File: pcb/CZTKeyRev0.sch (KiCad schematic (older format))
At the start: 268 parts, among them U1 proton_c

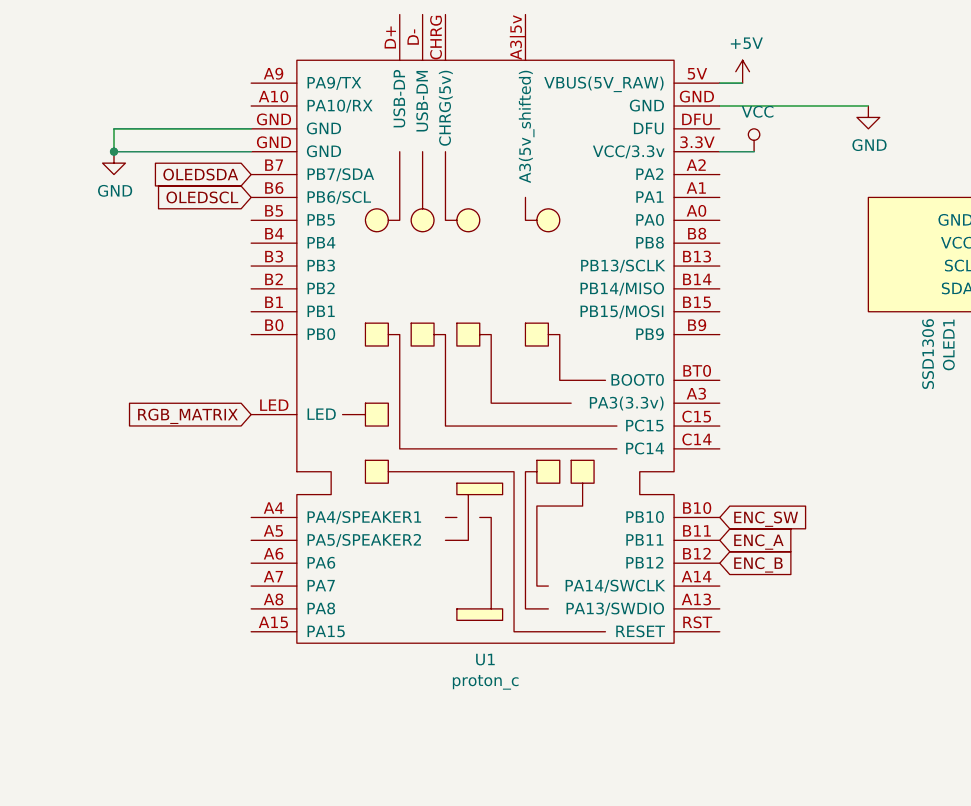
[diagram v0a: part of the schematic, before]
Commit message: Maybe final?
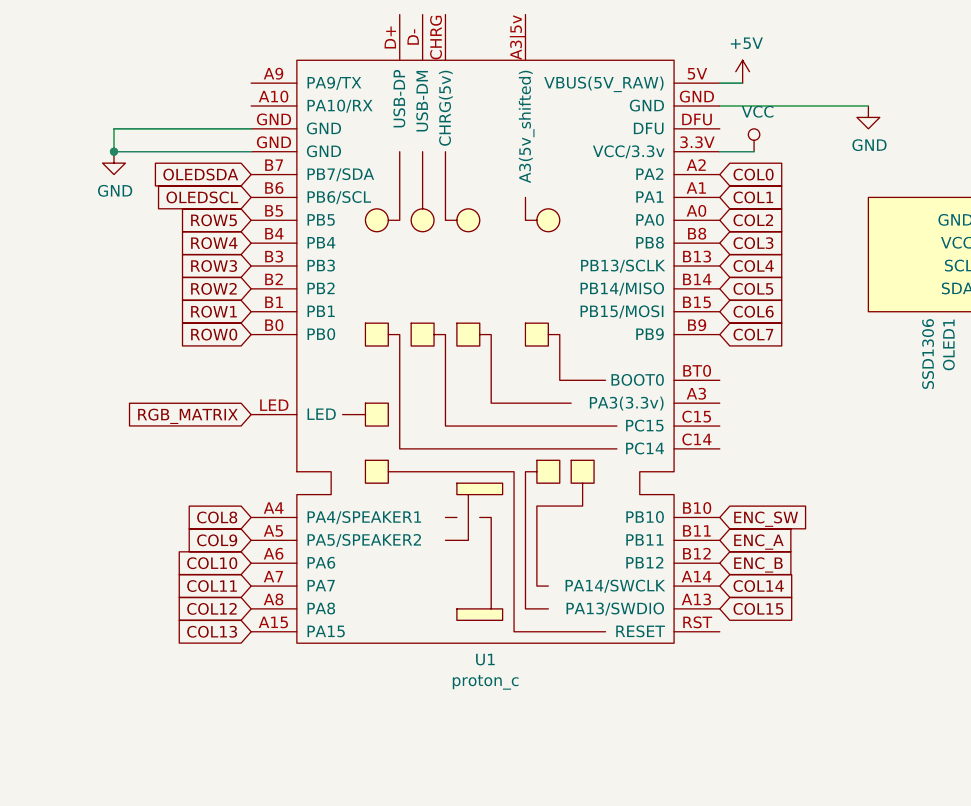
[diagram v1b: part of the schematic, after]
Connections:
- net COL0: now also U1.A2 (PA2)
- net COL1: now also U1.A1 (PA1)
- net COL10: now also U1.A6 (PA6)
- net COL11: now also U1.A7 (PA7)
- net COL12: now also U1.A8 (PA8)
- net COL13: now also U1.A15 (PA15)
- net COL14: now also U1.A14 (PA14/SWCLK)
- net COL15: now also U1.A13 (PA13/SWDIO)
- net COL2: now also U1.A0 (PA0)
- net COL3: now also U1.B8 (PB8)
- net COL4: now also U1.B13 (PB13/SCLK)
- net COL5: now also U1.B14 (PB14/MISO)
- net COL6: now also U1.B15 (PB15/MOSI)
- net COL7: now also U1.B9 (PB9)
- net COL8: now also U1.A4 (PA4/SPEAKER1)
- net COL9: now also U1.A5 (PA5/SPEAKER2)
- net ROW0: now also U1.B0 (PB0)
- net ROW1: now also U1.B1 (PB1)
- net ROW2: now also U1.B2 (PB2)
- net ROW3: now also U1.B3 (PB3)
- net ROW4: now also U1.B4 (PB4)
- net ROW5: now also U1.B5 (PB5)
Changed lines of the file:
@@
 Text GLabel 3250 2950 2    50   Input ~ 0
 ENC_SW
+Text GLabel 1200 2050 0    50   Input ~ 0
+ROW1
+Text GLabel 1200 2150 0    50   Input ~ 0
+ROW0
+Text GLabel 1200 1950 0    50   Input ~ 0
+ROW2
+Text GLabel 1200 1850 0    50   Input ~ 0
+ROW3
+Text GLabel 1200 1750 0    50   Input ~ 0
+ROW4
+Text GLabel 1200 1650 0    50   Input ~ 0
+ROW5
+Text GLabel 3250 1750 2    50   Input ~ 0
+COL3
+Text GLabel 3250 1650 2    50   Input ~ 0
+COL2
+Text GLabel 3250 1550 2    50   Input ~ 0
+COL1
+Text GLabel 3250 1450 2    50   Input ~ 0
+COL0
+Text GLabel 3250 1850 2    50   Input ~ 0
+COL4
+Text GLabel 3250 1950 2    50   Input ~ 0
+COL5
+Text GLabel 3250 2050 2    50   Input ~ 0
+COL6
+Text GLabel 3250 2150 2    50   Input ~ 0
+COL7
+Text GLabel 1200 2950 0    50   Input ~ 0
+COL8
+Text GLabel 1200 3050 0    50   Input ~ 0
+COL9
+Text GLabel 1200 3150 0    50   Input ~ 0
+COL10
+Text GLabel 1200 3250 0    50   Input ~ 0
+COL11
+Text GLabel 1200 3350 0    50   Input ~ 0
+COL12
+Text GLabel 1200 3450 0    50   Input ~ 0
+COL13
+Text GLabel 3250 3250 2    50   Input ~ 0
+COL14
+Text GLabel 3250 3350 2    50   Input ~ 0
+COL15
 $EndSCHEMATC

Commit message: did some stuff
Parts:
- added WS87: WS2812B, WS2812B-edited:Neopixel_easy_LED_WS2812B_PLCC4_5.0x5.0mm_P3.2mm, symbol LED:WS2812B
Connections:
- net +5V: now also WS87.1 (VDD)
- net GND: now also WS87.3 (VSS)
- net at WS83.4 (DIN): now also WS87.2 (DOUT); no longer WS82.2 (DOUT)
- new net: WS82.2 (DOUT), WS87.4 (DIN)
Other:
- moved on the sheet: C1, C2, D1, D10, D11, D12, D13, D14, D15, D16, D17, D18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
